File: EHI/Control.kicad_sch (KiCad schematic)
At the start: 15 parts

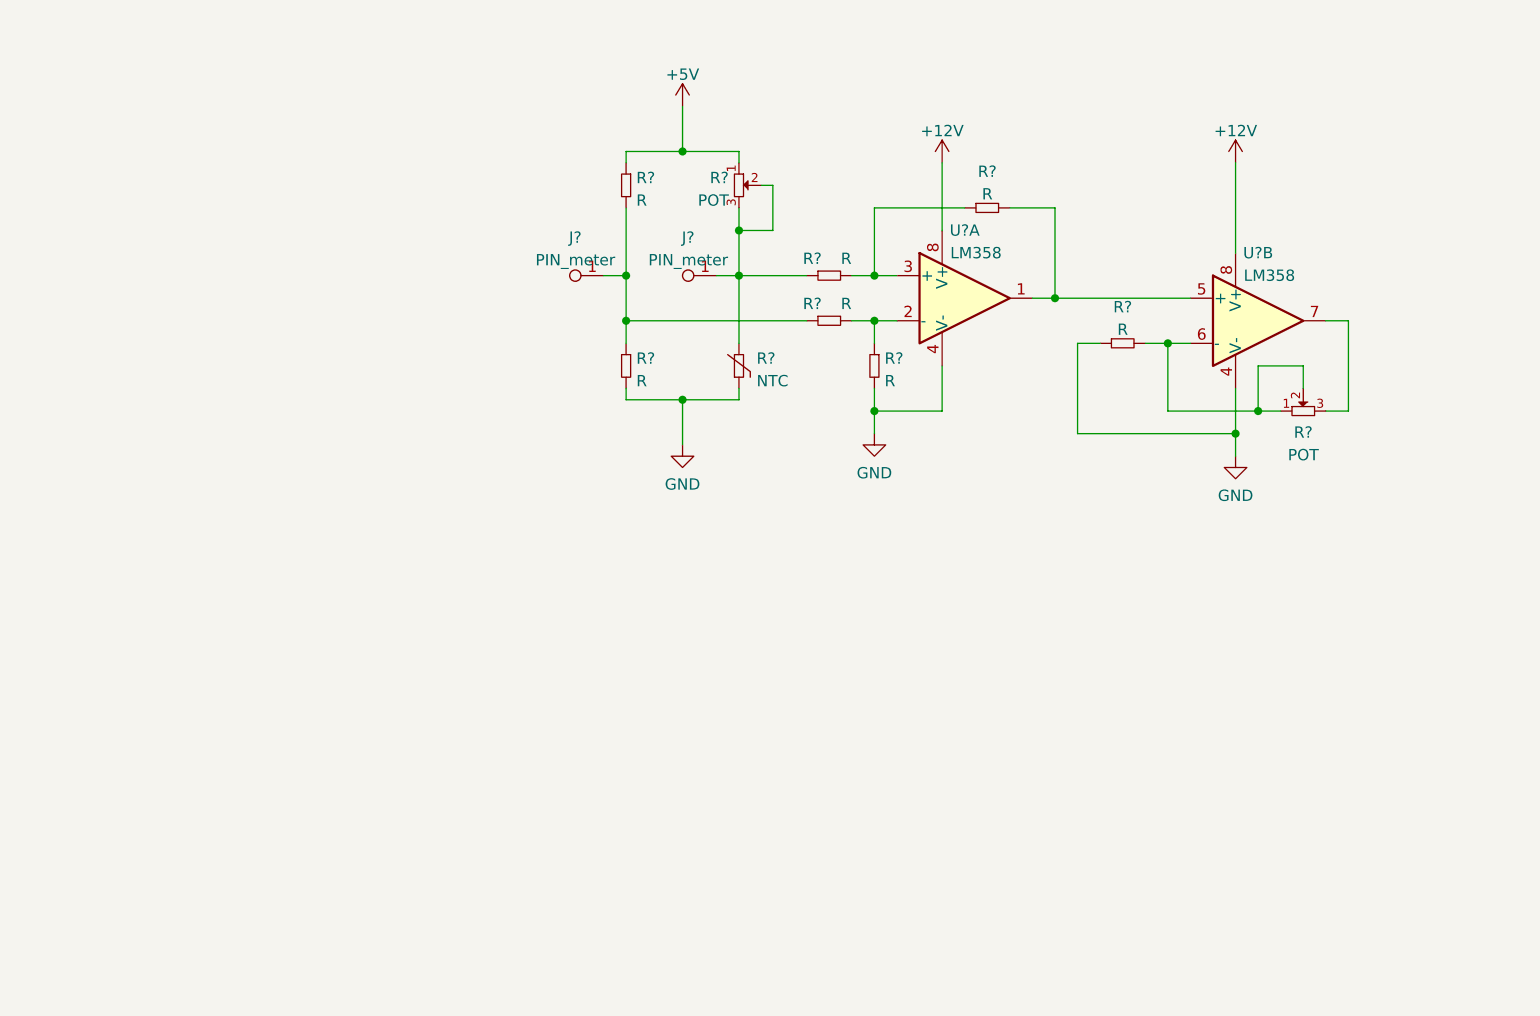
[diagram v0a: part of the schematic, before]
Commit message: actualizacion del proteyecto Olimpiadas
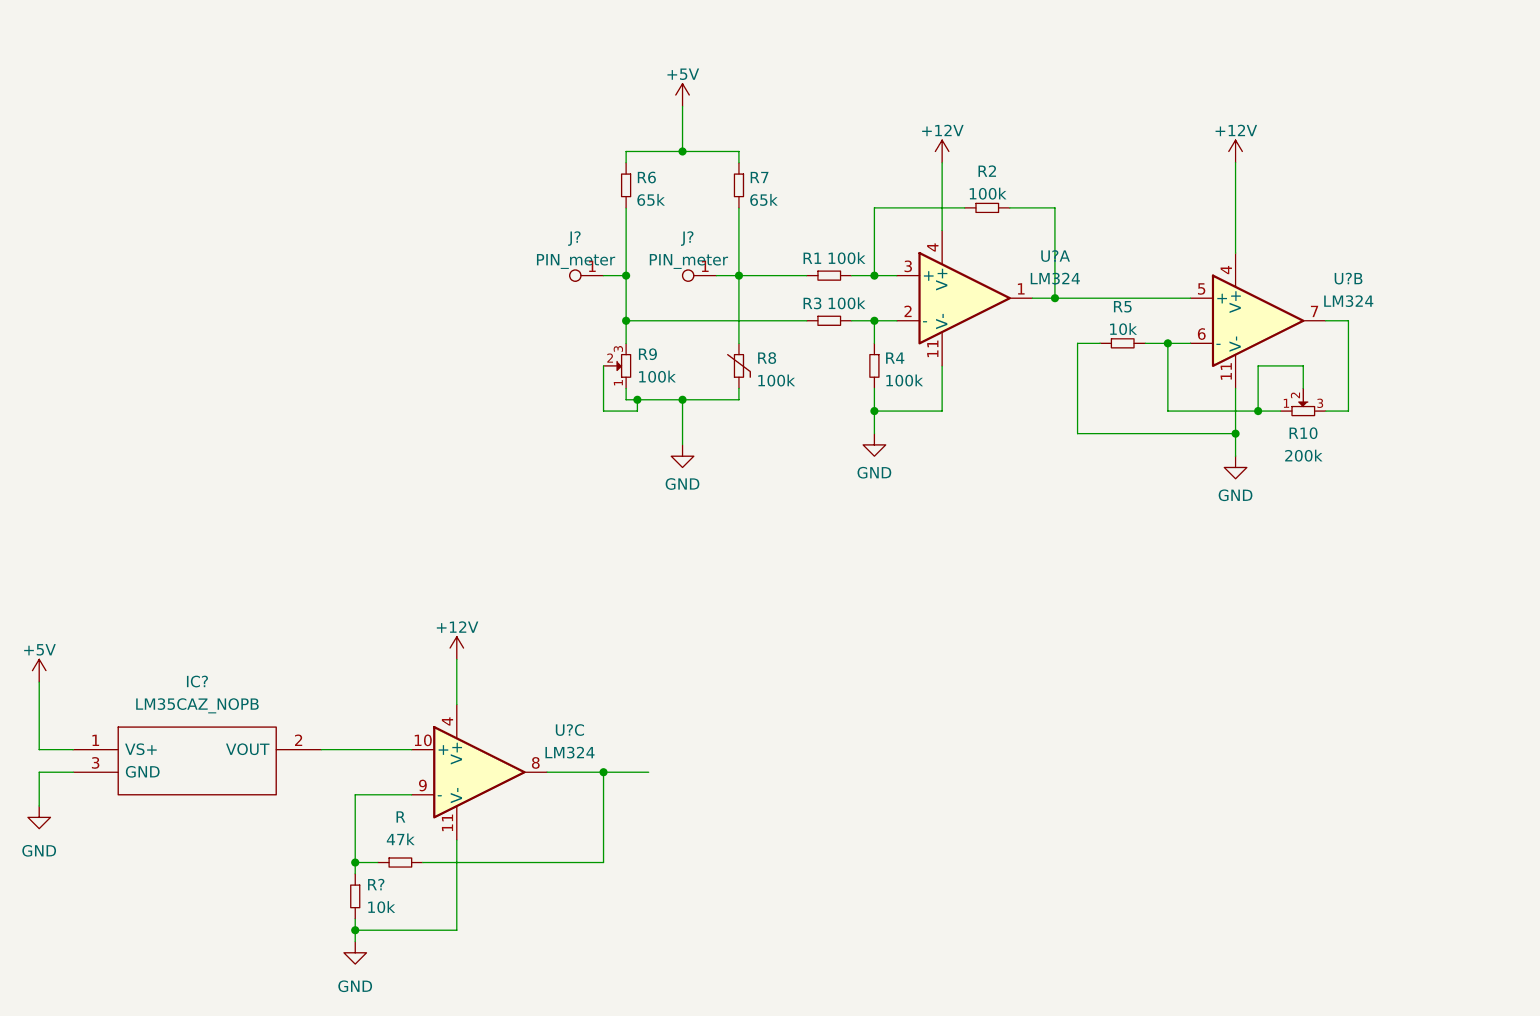
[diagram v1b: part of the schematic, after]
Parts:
- removed U? (x2): LM358, symbol MacroLib:LM358
- added IC?: LM35CAZ_NOPB, LP0003A, symbol MacroLib:LM35CAZ_NOPB
- added R: 47k, symbol EESTN5:R
- added R?: 10k, symbol EESTN5:R
- added U? (x3): LM324, symbol MacroLib:LM324
- R1, R2, R3, R4: renamed from R?; value R -> 100k
- R10: renamed from R?; value POT -> 200k
- R5: renamed from R?; value R -> 10k
- R6, R7: renamed from R?; value R -> 65k
- R8: renamed from R?; value NTC -> 100k
- R9: renamed from R?; value POT -> 100k
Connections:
- net +12V: now also U?.4 (V+), U?.4 (V+), U?.4 (V+)
- net +5V: now also R7.1, IC?.1 (VS+); no longer R9.1
- net GND: now also R9.1, R9.2, IC?.3 (GND), R?.2, U?.11 (V-), U?.11 (V-), U?.11 (V-); no longer R7.2
- net at J?.1, R3.1, R6.2: now also R9.3; no longer R7.1
- net at R3.2, R4.1: now also U?.2 (-)
- net at J?.1, R1.1, R8.2: now also R7.2; no longer R9.2, R9.3
- net at R2.2: now also U?.1, U?.5 (+)
- net at R1.2, R2.1: now also U?.3 (+)
- net at R10.1, R10.2, R5.2: now also U?.6 (-)
- net at R10.3: now also U?.7
- new net: R.1, R?.1, U?.9 (-)
- new net: IC?.2 (VOUT), U?.10 (+)
- new net: R.2, U?.8
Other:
- moved on the sheet: R7, R9

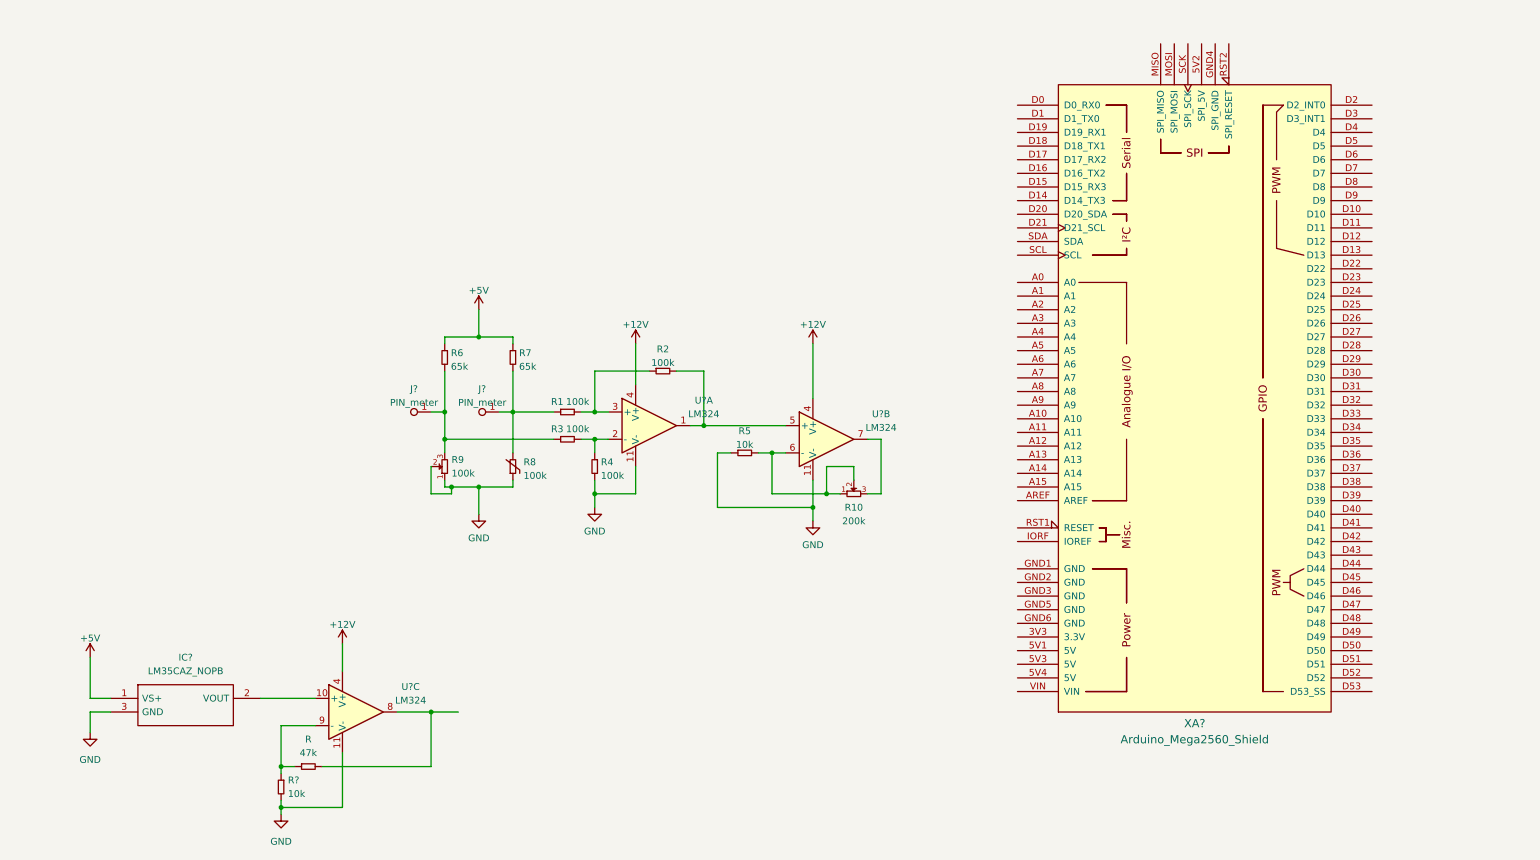
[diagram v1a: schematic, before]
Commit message: new
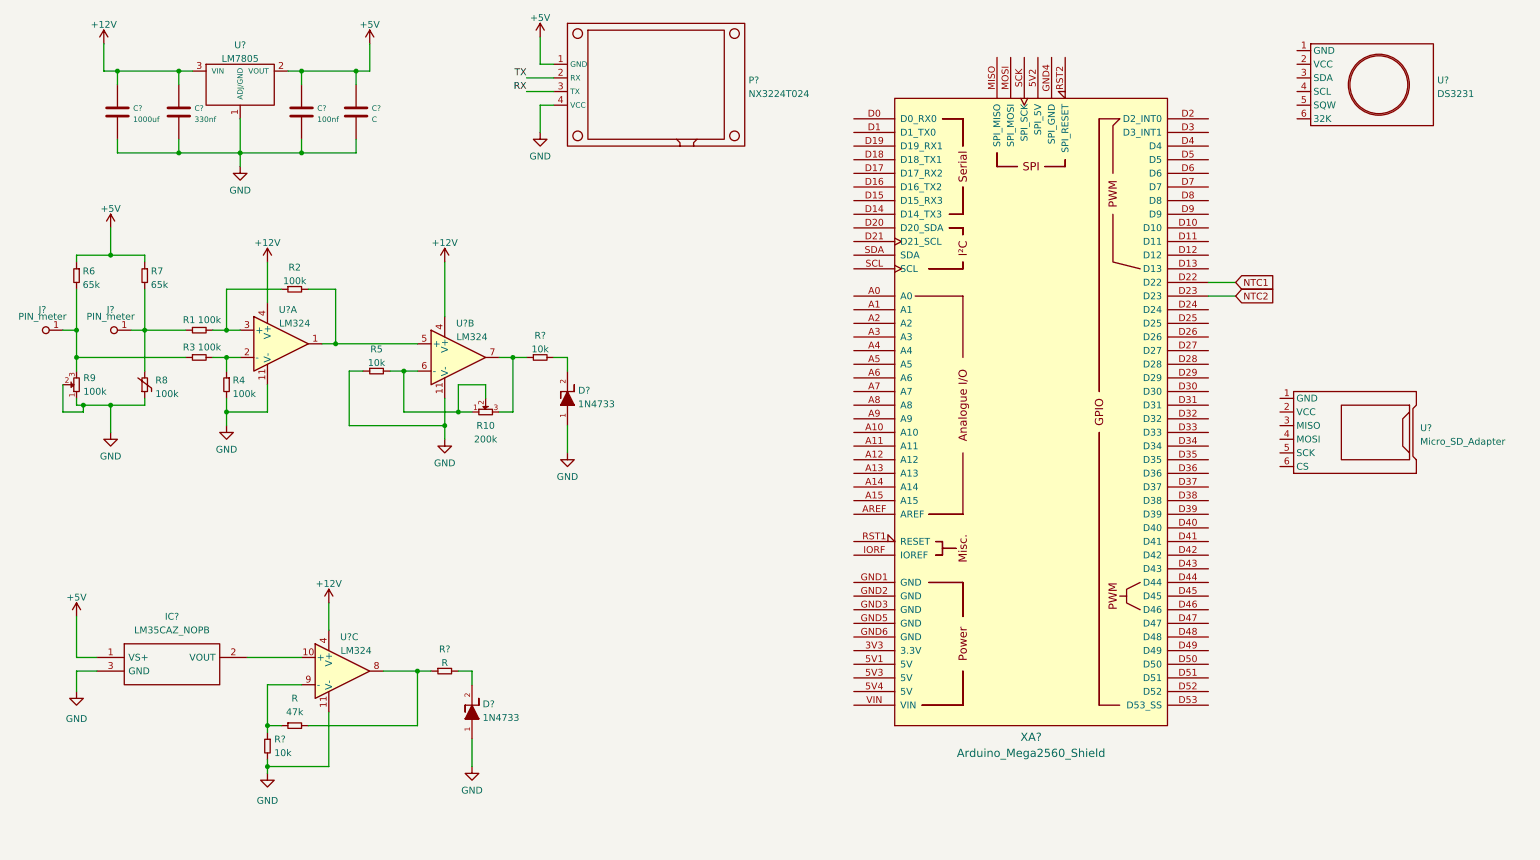
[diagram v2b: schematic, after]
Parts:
- added C?: C, symbol EESTN5:C
- added C?: 330nf, symbol EESTN5:C
- added C?: 1000uf, symbol EESTN5:C
- added C?: 100nf, symbol EESTN5:C
- added D? (x2): 1N4733, symbol MacroLib:ZENNER
- added P?: NX3224T024, symbol MacroLib:NX3224T024
- added R?: 10k, symbol EESTN5:R
- added R?: R, symbol EESTN5:R
- added U?: LM7805, symbol MacroLib:LM78XX
- added U?: Micro_SD_Adapter, symbol MacroLib:Micro_SD_Adapter
- added U?: DS3231, symbol MacroLib:DS3231
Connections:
- net +12V: now also C?.1, C?.1, U?.3 (VIN)
- net +5V: now also C?.1, C?.1, P?.1 (GND), U?.2 (VOUT)
- net GND: now also C?.2, C?.2, C?.2, C?.2, D?.1 (A), D?.1 (A), P?.4 (VCC), U?.1 (ADJ/GND)
- net NTC1: now reaches XA?.D22
- net NTC2: now reaches XA?.D23
- net at R10.3, U?.7: now also R?.1
- net at R.2, U?.8: now also R?.1
- new net: D?.2 (K), R?.2 (x2)
- new net RX: P?.3 (TX)
- new net TX: P?.2 (RX)
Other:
- moved on the sheet: IC?, J?, R, R1, R10, R2, R3, R4, R5, R6, R7, R8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
